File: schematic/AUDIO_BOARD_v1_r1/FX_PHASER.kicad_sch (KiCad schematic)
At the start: 43 parts, among them U50 LM13700, U51 LM13700, U52 OPA1678, U53 OPA1678, U54 OPA1678

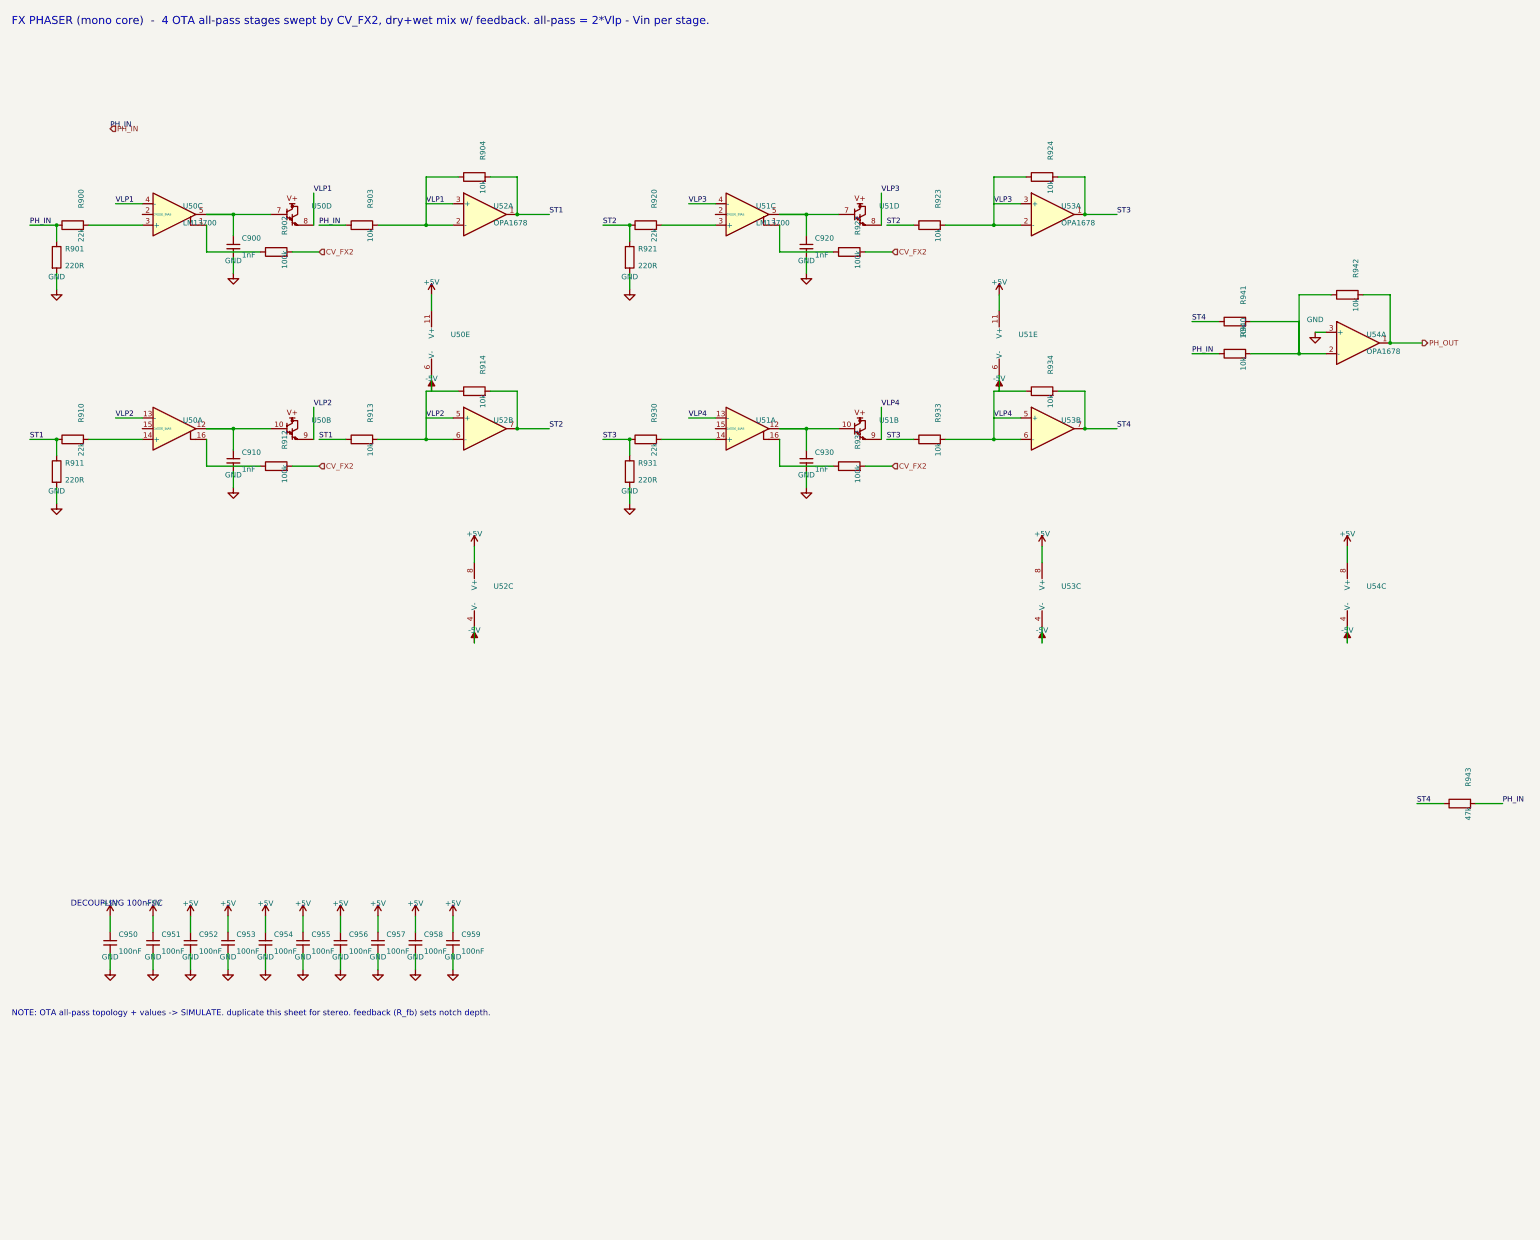
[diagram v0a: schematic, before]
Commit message: phaser? schematic is messy
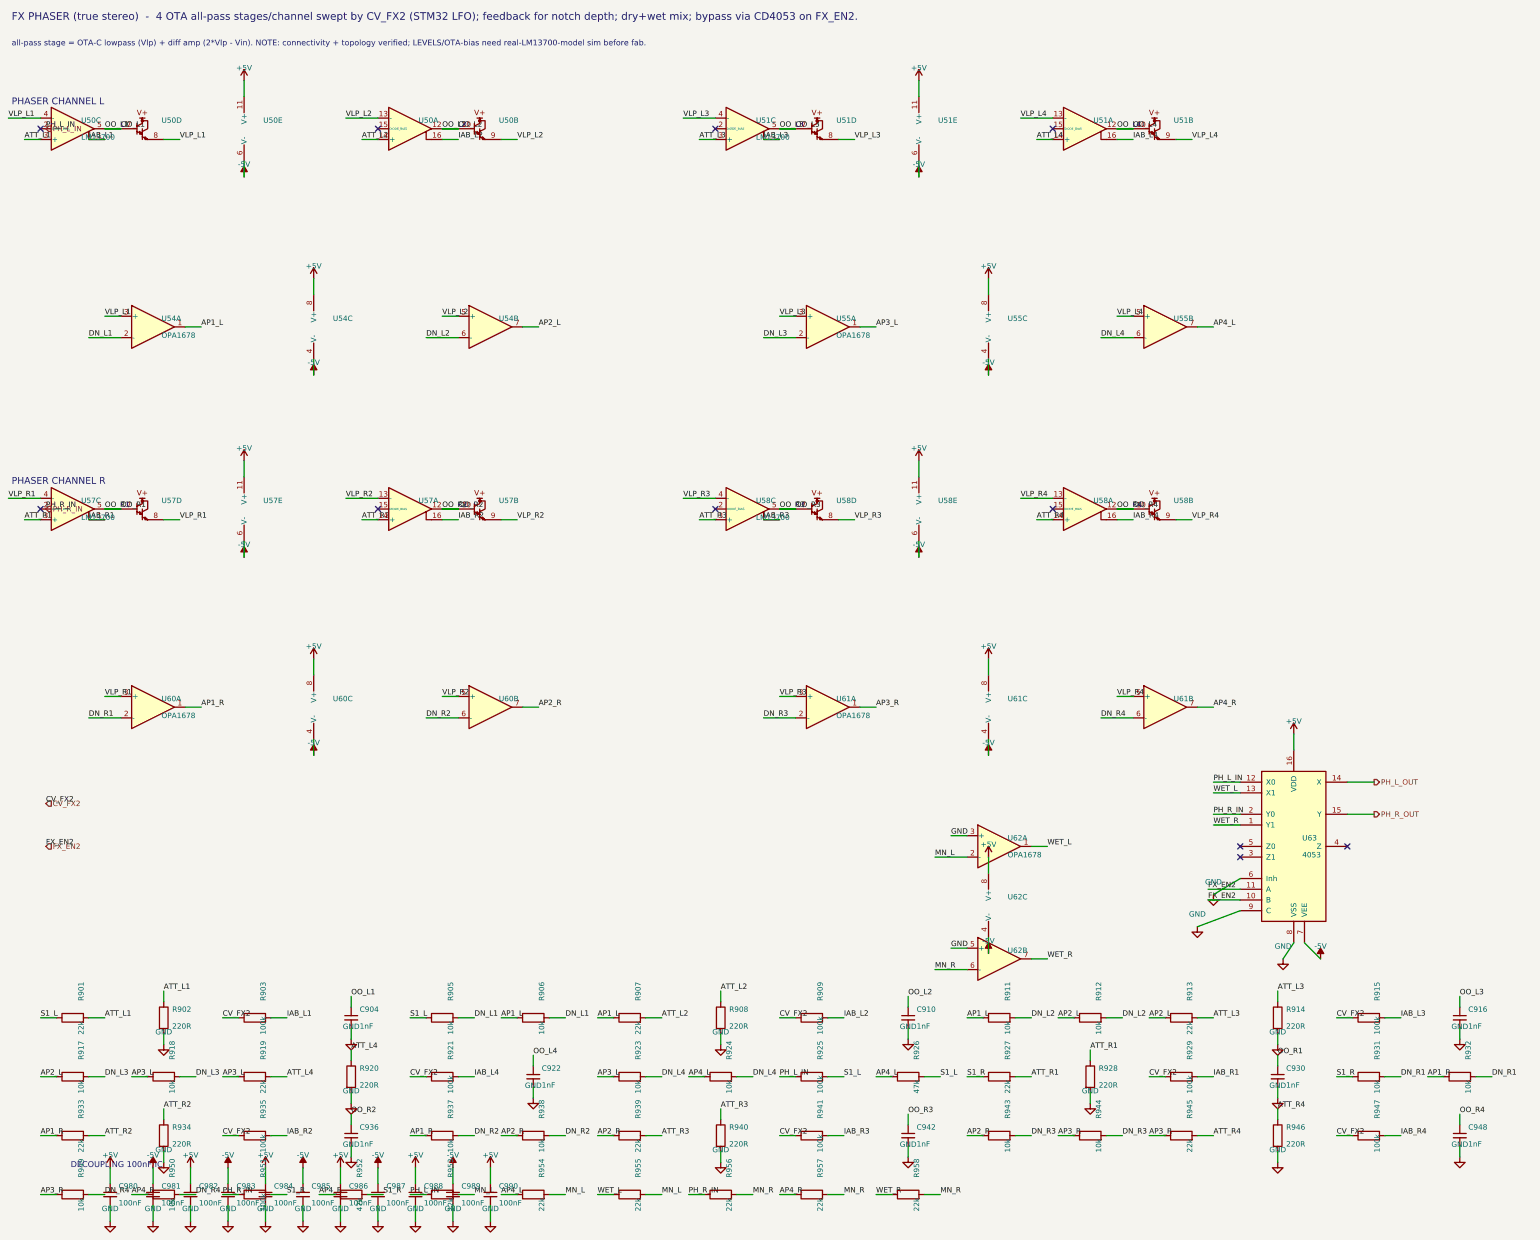
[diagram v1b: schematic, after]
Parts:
- removed C900, C920: 1nF, Capacitor_SMD:C_0402_1005Metric, symbol Device:C_Small
- removed C950, C951, C952, C953, C954, C955, C956, C957, C958, C959: 100nF, Capacitor_SMD:C_0402_1005Metric, symbol Device:C_Small
- removed R900, R910, R930: 22k, Resistor_SMD:R_0402_1005Metric, symbol Device:R
- removed R904, R942: 10k, Resistor_SMD:R_0402_1005Metric, symbol Device:R
- removed R922: 100k, Resistor_SMD:R_0402_1005Metric, symbol Device:R
- removed U52, U53: OPA1678, Package_DIP:DIP-8_W7.62mm_SMDSocket_SmallPads, symbol Amplifier_Operational:OPA1678
- added C904, C916, C922, C936, C942, C948: 1nF, Capacitor_SMD:C_0402_1005Metric, symbol Device:C_Small
- added C980, C981, C982, C983, C984, C985, C986, C987, C988, C989, C990: 100nF, Capacitor_SMD:C_0402_1005Metric, symbol Device:C_Small
- added R905, R906, R917, R918, R937, R938, R944, R949, R950: 10k, Resistor_SMD:R_0402_1005Metric, symbol Device:R
- added R907, R919, R927, R939, R945, R953, R954, R955, R956, R957, R958: 22k, Resistor_SMD:R_0402_1005Metric, symbol Device:R
- added R908, R928, R946: 220R, Resistor_SMD:R_0402_1005Metric, symbol Device:R
- added R909, R915, R925, R929, R935, R947, R951: 100k, Resistor_SMD:R_0402_1005Metric, symbol Device:R
- added R926, R952: 47k, Resistor_SMD:R_0402_1005Metric, symbol Device:R
- added unit 2 of U54
- added U55, U61: OPA1678, symbol Amplifier_Operational:OPA1678
- added U57, U58: LM13700, symbol Amplifier_Operational:LM13700
- added U60, U62: OPA1678, Package_DIP:DIP-8_W7.62mm_SMDSocket_SmallPads, symbol Amplifier_Operational:OPA1678
- added U63: 4053, Package_SO:SOIC-16_3.9x9.9mm_P1.27mm, symbol 4xxx:4053
- R901: value 220R -> 22k
- R902: value 100k -> 220R
- R903, R941: value 10k -> 100k
- R911, R931: value 220R -> 10k
- R912, R932: value 100k -> 10k
- R913, R933: value 10k -> 22k
- R914, R934, R940: value 10k -> 220R
- R920: value 22k -> 220R
- R921: value 220R -> 100k
- R943: value 47k -> 10k
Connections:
- net +5V: now also C980.1, C982.1, C984.1, C986.1, C988.1, C990.1, U55.8 (V+), U57.11 (V+), U58.11 (V+), U60.8 (V+), U61.8 (V+), U62.8 (V+), U63.16 (VDD)
- net -5V: now also C981.1, C983.1, C985.1, C987.1, C989.1, U55.4 (V-), U57.6 (V-), U58.6 (V-), U60.4 (V-), U61.4 (V-), U62.4 (V-), U63.7 (VEE)
- net CV_FX2: now also R903.1, R921.1, R941.1, R909.1, R915.1, R929.1, R935.1, R947.1; no longer R902.2, R912.2, R932.2
- net GND: now also R902.2, R914.2, R920.2, R934.2, R940.2, C904.2, C916.2, C922.2, C936.2, C942.2, C948.2, C980.2, C981.2, C982.2, C983.2, C984.2, C985.2, C986.2, C987.2, C988.2, C989.2, C990.2, R908.2, R928.2, R946.2, U62.3 (+), U62.5 (+), U63.6 (Inh), U63.8 (VSS), U63.9 (C); no longer R901.2, R911.2, R921.2, R931.2, U54.3 (+)
- net OO_L1: now reaches U50.5, U50.7
- net OO_L1: now also C904.1
- net ATT_L1: now reaches U50.3 (+)
- net ATT_L1: now also R901.2, R902.1
- net IAB_L1: now reaches U50.1
- net IAB_L1: now also R903.2; no longer R902.1
- net ATT_L4: now reaches U51.14 (+)
- net ATT_L4: now also R920.1, R919.2
- net OO_L4: now reaches U51.10, U51.12
- net OO_L4: now also C922.1; no longer C930.1
- net AP2_L: now reaches R912.1
- net AP2_L: now also R913.1, R917.1, U54.7; no longer U50.16
- net AP1_R: now reaches R932.1
- net AP1_R: now also R933.1, R937.1, U60.1; no longer U51.16
- net IAB_L3: now reaches U51.1
- net IAB_L3: now also R915.2
- net ATT_L3: now reaches U51.3 (+)
- net ATT_L3: now also R913.2, R914.1; no longer R920.2
- net OO_L3: now reaches U51.5, U51.7
- net OO_L3: now also C916.1
- net OO_L2: now reaches C910.1, U50.10, U50.12
- net ATT_L2: now reaches U50.14 (+)
- net ATT_L2: now also R907.2, R908.1
- removed net PH_IN: R901.1, R903.1, R940.1, R943.2
- net PH_OUT renamed AP1_L
- net AP1_L: now also R911.1, R906.1, R907.1
- removed net ST1: R911.1, R913.1
- removed net ST2: R914.2, R920.1, R921.1, R923.1
- removed net ST3: R924.2, R931.1, R933.1
- removed net ST4: R934.2, R941.1, R943.1
- net VLP1 renamed VLP_L1
- net VLP_L1: now also U54.3 (+); no longer R903.2
- net VLP2 renamed VLP_L2
- net VLP_L2: now also U54.5 (+); no longer R913.2, R914.1
- net VLP3 renamed VLP_L3
- net VLP_L3: now also U55.3 (+); no longer R923.2, R924.1
- net VLP4 renamed ATT_R2
- net ATT_R2: now also U57.14 (+); no longer U51.13 (-), U51.9
- new net AP2_R: R938.1, R939.1, R943.1, U60.7
- new net AP3_L: R918.1, R919.1, R923.1, U55.1
- new net AP3_R: R944.1, R945.1, R949.1, U61.1
- new net AP4_L: R924.1, R926.1, R954.1, U55.7
- new net AP4_R: R950.1, R952.1, R957.1, U61.7
- new net ATT_R1: R927.2, R928.1, U57.3 (+)
- new net ATT_R3: R939.2, R940.1, U58.3 (+)
- new net ATT_R4: R945.2, R946.1, U58.14 (+)
- new net DN_L1: R905.2, R906.2, U54.2 (-)
- new net DN_L2: R911.2, R912.2, U54.6 (-)
- new net DN_L3: R917.2, R918.2, U55.2 (-)
- new net DN_L4: R923.2, R924.2, U55.6 (-)
- new net DN_R1: R931.2, R932.2, U60.2 (-)
- new net DN_R2: R937.2, R938.2, U60.6 (-)
- new net DN_R3: R943.2, R944.2, U61.2 (-)
- new net DN_R4: R949.2, R950.2, U61.6 (-)
- new net FX_EN2: U63.10 (B), U63.11 (A)
- new net IAB_L2: R909.2, U50.16
- new net IAB_L4: R921.2, U51.16
- new net IAB_R1: R929.2, U57.1
- new net IAB_R2: R935.2, U57.16
- new net IAB_R3: R941.2, U58.1
- new net IAB_R4: R947.2, U58.16
- new net MN_L: R953.2, R954.2, R955.2, U62.2 (-)
- new net MN_R: R956.2, R957.2, R958.2, U62.6 (-)
- new net OO_R1: C930.1, U57.5, U57.7
- new net OO_R2: C936.1, U57.10, U57.12
- new net OO_R3: C942.1, U58.5, U58.7
- new net OO_R4: C948.1, U58.10, U58.12
- new net PH_L_IN: R925.1, R953.1, U63.12 (X0)
- new net PH_L_OUT: U63.14 (X)
- new net PH_R_IN: R951.1, R956.1, U63.2 (Y0)
- new net PH_R_OUT: U63.15 (Y)
- new net S1_L: R901.1, R905.1, R925.2, R926.2
- new net S1_R: R927.1, R931.1, R951.2, R952.2
- new net VLP_L4: U51.13 (-), U51.9, U55.5 (+)
- new net VLP_R1: U57.4 (-), U57.8, U60.3 (+)
- new net VLP_R2: U57.13 (-), U57.9, U60.5 (+)
- new net VLP_R3: U58.4 (-), U58.8, U61.3 (+)
- new net VLP_R4: U58.13 (-), U58.9, U61.5 (+)
- new net WET_L: R955.1, U62.1, U63.13 (X1)
- new net WET_R: R958.1, U62.7, U63.1 (Y1)
- no-connect marks 0 -> 11
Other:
- note added: "FX PHASER (true stereo) - 4 OTA all-pass stages/channel swept by CV_FX2 (STM32 LFO); feedback for notch depth; dry+wet mix; bypass via CD4053 on FX_EN2."
- note added: "PHASER CHANNEL L"
- note added: "PHASER CHANNEL R"
- note added: "all-pass stage = OTA-C lowpass (Vlp) + diff amp (2*Vlp - Vin). NOTE: connectivity + topology verified; LEVELS/OTA-bias need real-LM13700-model sim before fab."
- note removed: "FX PHASER (mono core) - 4 OTA all-pass stages swept by CV_FX2, dry+wet mix w/ feedback. all-pass = 2*Vlp - Vin per stage."
- note removed: "NOTE: OTA all-pass topology + values -> SIMULATE. duplicate this sheet for stereo. feedback (R_fb) sets notch depth."

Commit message: sim, render, audio stuff
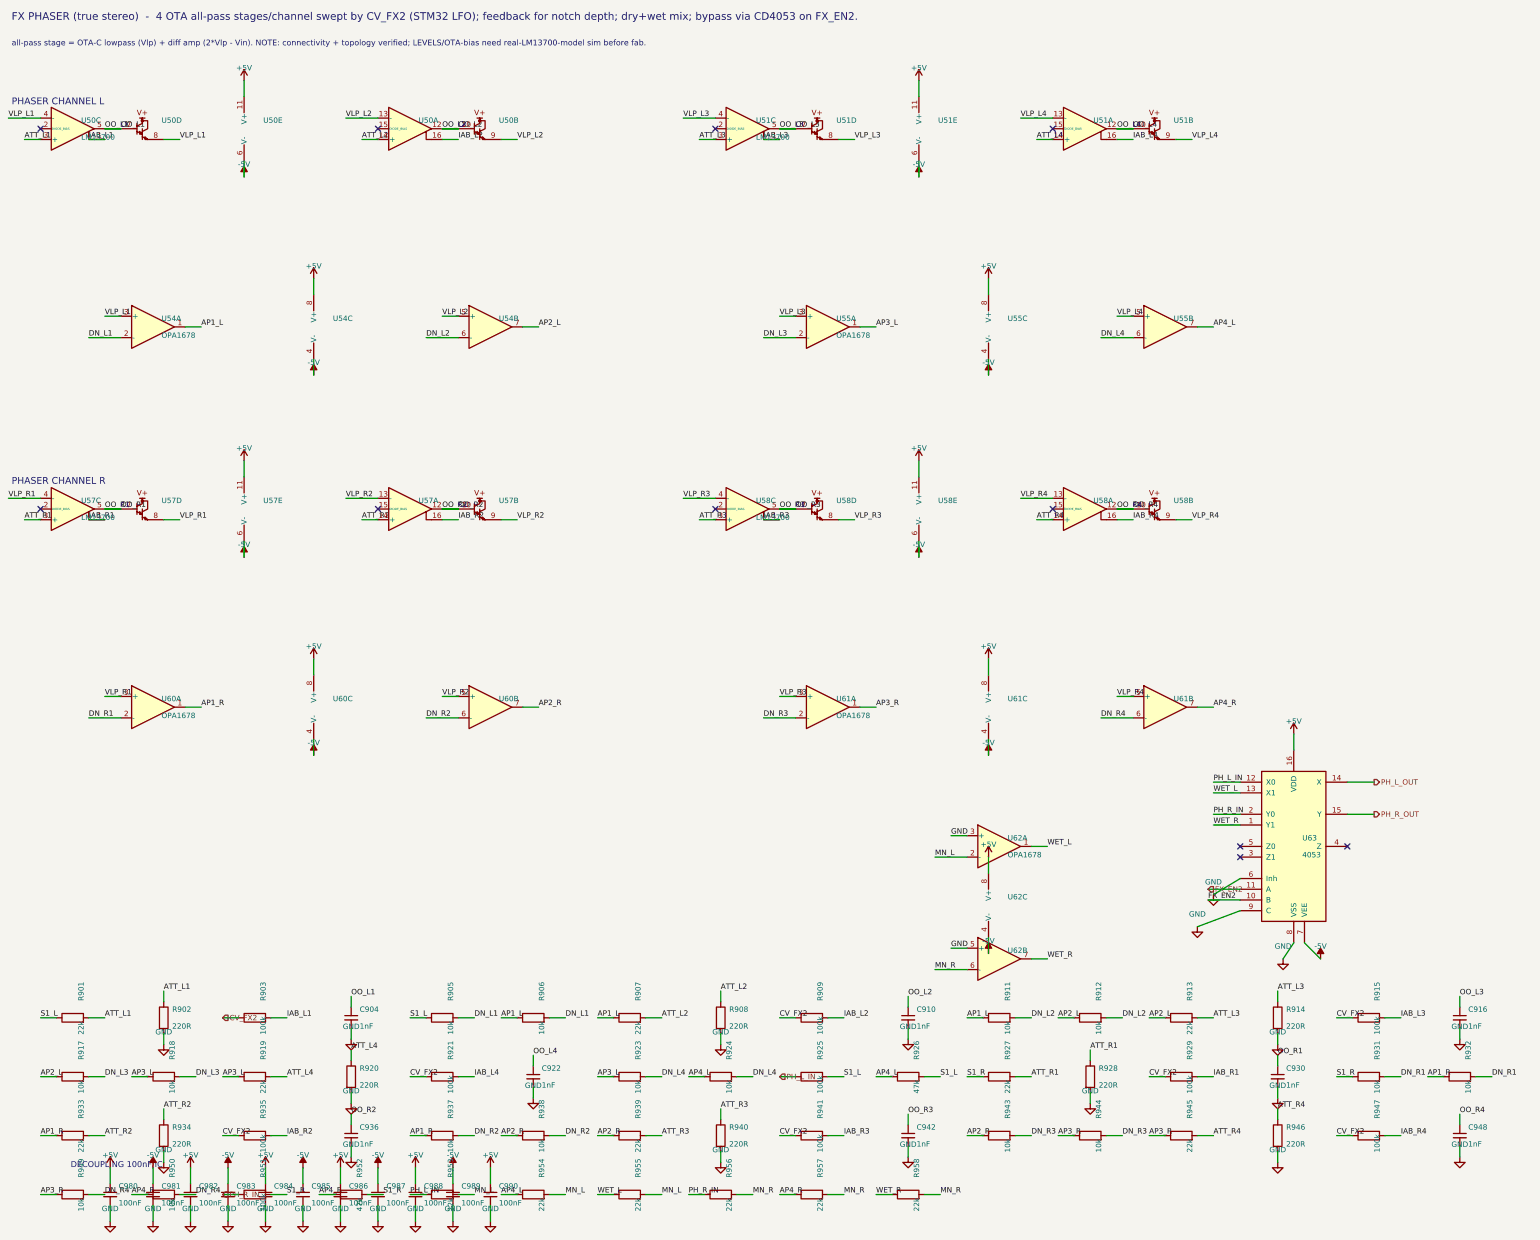
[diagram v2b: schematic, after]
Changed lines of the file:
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@@
 		(instances (project "AUDIO_BOARD" (path "/ba93534c-f2e3-4dc0-9a76-585fdc68cf39/aa11bb22-cc33-dd44-ee55-ff6677889900" (reference "R903") (unit 1)))))
 	(wire (pts (xy 69.85 250.19) (xy 66.04 250.19)) (stroke (width 0) (type default)))
-	(label "CV_FX2" (at 66.04 250.19 0) (effects (font (size 1.27 1.27)) (justify left bottom)))
+	(hierarchical_label "CV_FX2" (shape input) (at 66.04 250.19 0) (effects (font (size 1.27 1.27)) (justify left)))
 	(wire (pts (xy 77.47 250.19) (xy 81.28 250.19)) (stroke (width 0) (type default)))
 	(label "IAB_L1" (at 81.28 250.19 0) (effects (font (size 1.27 1.27)) (justify left bottom)))
@@
 		(instances (project "AUDIO_BOARD" (path "/ba93534c-f2e3-4dc0-9a76-585fdc68cf39/aa11bb22-cc33-dd44-ee55-ff6677889900" (reference "R925") (unit 1)))))
 	(wire (pts (xy 201.93 264.16) (xy 198.12 264.16)) (stroke (width 0) (type default)))
-	(label "PH_L_IN" (at 198.12 264.16 0) (effects (font (size 1.27 1.27)) (justify left bottom)))
+	(hierarchical_label "PH_L_IN" (shape input) (at 198.12 264.16 0) (effects (font (size 1.27 1.27)) (justify left)))
 	(wire (pts (xy 209.55 264.16) (xy 213.36 264.16)) (stroke (width 0) (type default)))
 	(label "S1_L" (at 213.36 264.16 0) (effects (font (size 1.27 1.27)) (justify left bottom)))
@@
 		(instances (project "AUDIO_BOARD" (path "/ba93534c-f2e3-4dc0-9a76-585fdc68cf39/aa11bb22-cc33-dd44-ee55-ff6677889900" (reference "R951") (unit 1)))))
 	(wire (pts (xy 69.85 292.1) (xy 66.04 292.1)) (stroke (width 0) (type default)))
-	(label "PH_R_IN" (at 66.04 292.1 0) (effects (font (size 1.27 1.27)) (justify left bottom)))
+	(hierarchical_label "PH_R_IN" (shape input) (at 66.04 292.1 0) (effects (font (size 1.27 1.27)) (justify left)))
 	(wire (pts (xy 77.47 292.1) (xy 81.28 292.1)) (stroke (width 0) (type default)))
 	(label "S1_R" (at 81.28 292.1 0) (effects (font (size 1.27 1.27)) (justify left bottom)))
@@
 	(hierarchical_label "PH_L_OUT" (shape output) (at 339.09 194.31 0) (effects (font (size 1.27 1.27)) (justify left)))
 	(wire (pts (xy 307.34 219.71) (xy 299.72 219.71)) (stroke (width 0) (type default)))
-	(label "FX_EN2" (at 299.72 219.71 0) (effects (font (size 1.27 1.27)) (justify left bottom)))
+	(hierarchical_label "FX_EN2" (shape input) (at 299.72 219.71 0) (effects (font (size 1.27 1.27)) (justify left)))
 	(wire (pts (xy 307.34 201.93) (xy 300.99 201.93)) (stroke (width 0) (type default)))
 	(label "PH_R_IN" (at 300.99 201.93 0) (effects (font (size 1.27 1.27)) (justify left bottom)))
@@
 		(property "Value" "-5V" (at 326.39 233.22 0) (effects (font (size 1.27 1.27))))
 		(instances (project "AUDIO_BOARD" (path "/ba93534c-f2e3-4dc0-9a76-585fdc68cf39/aa11bb22-cc33-dd44-ee55-ff6677889900" (reference "#PWR939") (unit 1)))))
-	(hierarchical_label "PH_L_IN" (shape input) (at 24.13 39.37 0) (effects (font (size 1.27 1.27)) (justify left)))
-	(label "PH_L_IN" (at 24.13 39.37 0) (effects (font (size 1.27 1.27)) (justify left bottom)))
-	(hierarchical_label "PH_R_IN" (shape input) (at 24.13 129.54 0) (effects (font (size 1.27 1.27)) (justify left)))
-	(label "PH_R_IN" (at 24.13 129.54 0) (effects (font (size 1.27 1.27)) (justify left bottom)))
-	(hierarchical_label "CV_FX2" (shape input) (at 24.13 199.39 0) (effects (font (size 1.27 1.27)) (justify left)))
-	(label "CV_FX2" (at 24.13 199.39 0) (effects (font (size 1.27 1.27)) (justify left bottom)))
-	(hierarchical_label "FX_EN2" (shape input) (at 24.13 209.55 0) (effects (font (size 1.27 1.27)) (justify left)))
-	(label "FX_EN2" (at 24.13 209.55 0) (effects (font (size 1.27 1.27)) (justify left bottom)))
 	(text "DECOUPLING 100nF/IC" (exclude_from_sim no) (at 30 286 0) (effects (font (size 1.4 1.4) ) (justify left bottom)))
 	(symbol (lib_id "Device:C_Small") (at 39.37 292.1 0) (unit 1)
@@
 	(no_connect
 		(at 22.86 39.37)
+		(uuid "dbFX0000-0000-0000-0000-000000000000")
 	)
 	(no_connect
 		(at 22.86 129.54)
+		(uuid "dbFX0000-0000-0000-0000-000000000001")
 	)
 	(no_connect
 		(at 102.87 39.37)
+		(uuid "dbFX0000-0000-0000-0000-000000000002")
 	)
 	(no_connect
 		(at 102.87 129.54)
+		(uuid "dbFX0000-0000-0000-0000-000000000003")
 	)
 	(no_connect
 		(at 182.88 39.37)
+		(uuid "dbFX0000-0000-0000-0000-000000000004")
 	)
 	(no_connect
 		(at 182.88 129.54)
+		(uuid "dbFX0000-0000-0000-0000-000000000005")
 	)
 	(no_connect
 		(at 262.89 39.37)
+		(uuid "dbFX0000-0000-0000-0000-000000000006")
 	)
 	(no_connect
 		(at 262.89 129.54)
+		(uuid "dbFX0000-0000-0000-0000-000000000007")
 	)
 	(no_connect
 		(at 307.34 209.55)
+		(uuid "dbFX0000-0000-0000-0000-000000000008")
 	)
 	(no_connect
 		(at 307.34 212.09)
+		(uuid "dbFX0000-0000-0000-0000-000000000009")
 	)
 	(no_connect
 		(at 332.74 209.55)
+		(uuid "dbFX0000-0000-0000-0000-000000000010")
 	)
 )
